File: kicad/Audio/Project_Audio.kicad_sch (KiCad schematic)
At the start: 9 parts, among them U1 PIC32MX170F256B, U2 Audio

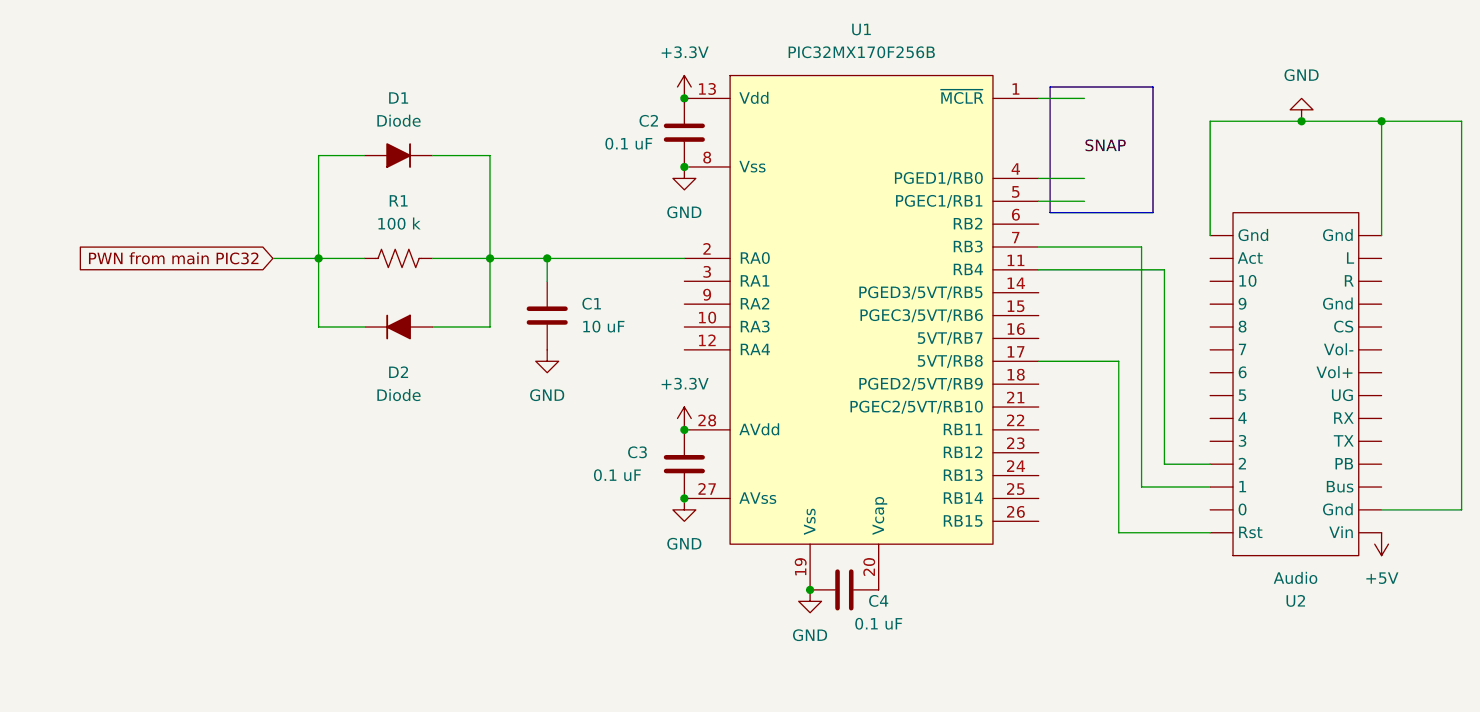
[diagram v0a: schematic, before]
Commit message: Revert to 3d98758
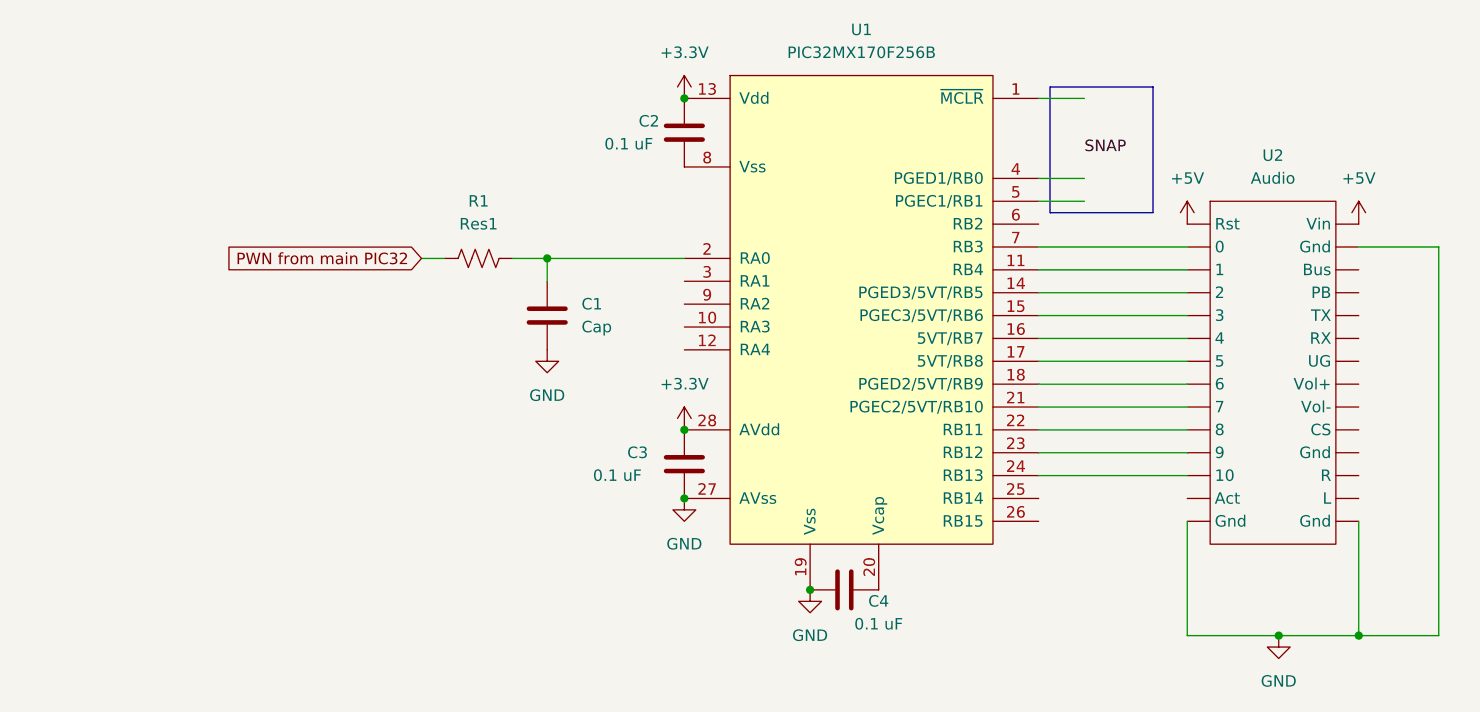
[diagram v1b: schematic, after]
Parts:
- removed D1, D2: Diode, symbol ME218_BaseLib:Diode
- C1: value 10 uF -> Cap
- R1: value 100 k -> Res1
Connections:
- net GND: no longer C2.2, U1.8 (Vss)
- net at U1.14 (PGED3/5VT/RB5): now also U2. (Vol-)
- net at U1.15 (PGEC3/5VT/RB6): now also U2. (Vol-)
- net at U1.16 (5VT/RB7): now also U2. (Vol-)
- net at U1.18 (PGED2/5VT/RB9): now also U2. (Vol-)
- net at U1.21 (PGEC2/5VT/RB10): now also U2. (Vol-)
- net at U1.22 (RB11): now also U2. (Vol-)
- net at U1.23 (RB12): now also U2. (Vol-)
- net at U1.24 (RB13): now also U2. (Vol-)
- new net: C2.2, U1.8 (Vss)
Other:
- moved on the sheet: R1, U2

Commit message: Update audio kicad
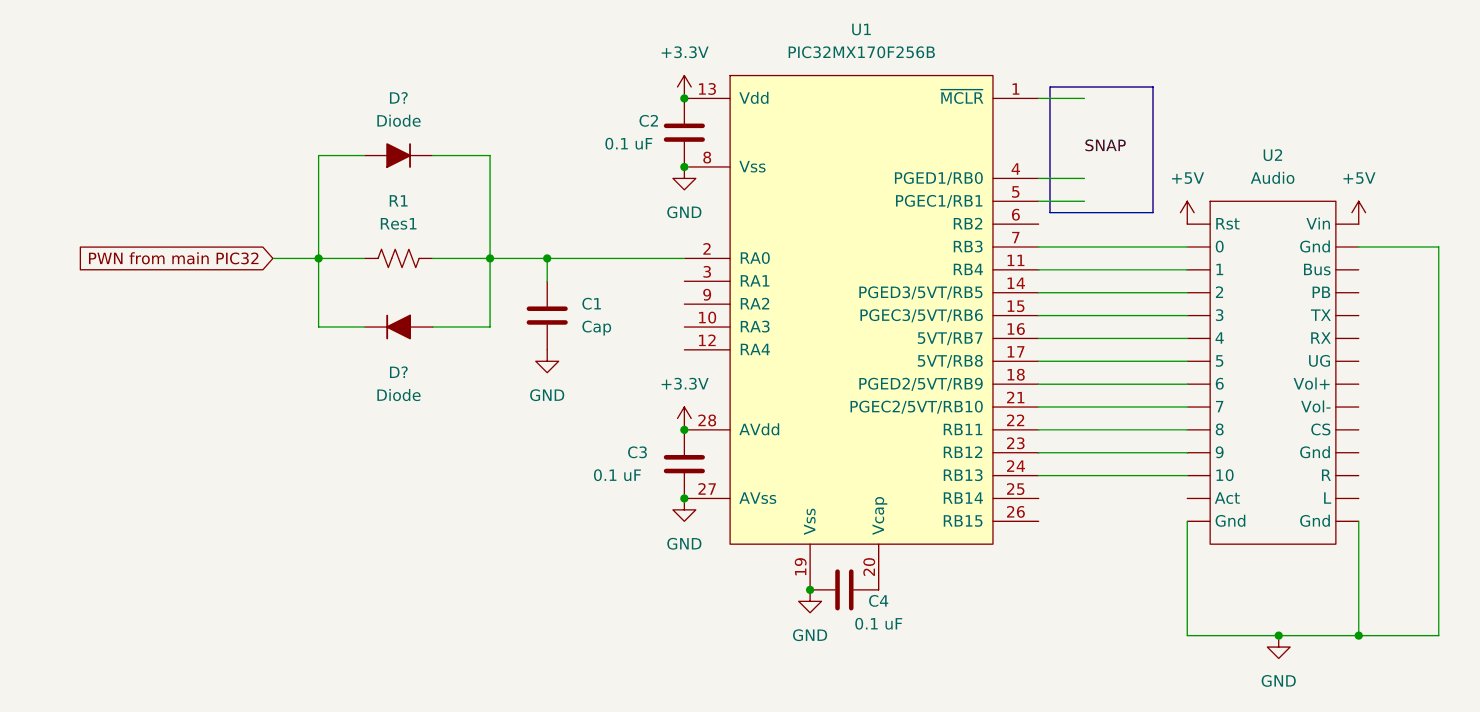
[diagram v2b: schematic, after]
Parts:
- added D? (x2): Diode, symbol ME218_BaseLib:Diode
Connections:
- net GND: now also C2.2, U1.8 (Vss)
- net PWN from main PIC32: now also D?.1 (K), D?.2 (A)
- net at C1.1, R1.2, U1.2 (RA0): now also D?.1 (K), D?.2 (A)
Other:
- moved on the sheet: R1
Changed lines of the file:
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@@
   (junction (at 69.85 85.09) (diameter 0) (color 0 0 0 0)
   )
+  (junction (at 63.5 85.09) (diameter 0) (color 0 0 0 0)
+  )
   (junction (at 85.09 111.76) (diameter 0) (color 0 0 0 0)
   )
@@
   (junction (at 151.13 127) (diameter 0) (color 0 0 0 0)
   )
+  (junction (at 44.45 85.09) (diameter 0) (color 0 0 0 0)
+  )
   (junction (at 85.09 104.14) (diameter 0) (color 0 0 0 0)
   )
@@
   (junction (at 85.09 67.31) (diameter 0) (color 0 0 0 0)
   )
+  (junction (at 85.09 74.93) (diameter 0) (color 0 0 0 0)
+  )
+  (wire (pts (xy 44.45 92.71) (xy 44.45 85.09))
+    (stroke (width 0) (type default) (color 0 0 0 0))
+  )
   (polyline (pts (xy 137.16 80.01) (xy 125.73 80.01))
     (stroke (width 0) (type default) (color 0 0 0 0))
@@
     (stroke (width 0) (type default) (color 0 0 0 0))
   )
-  (wire (pts (xy 55.88 85.09) (xy 58.42 85.09))
+  (wire (pts (xy 39.37 85.09) (xy 44.45 85.09))
     (stroke (width 0) (type default) (color 0 0 0 0))
   )
@@
     (stroke (width 0) (type default) (color 0 0 0 0))
   )
-  (wire (pts (xy 66.04 85.09) (xy 69.85 85.09))
+  (wire (pts (xy 57.15 85.09) (xy 63.5 85.09))
+    (stroke (width 0) (type default) (color 0 0 0 0))
+  )
+  (wire (pts (xy 63.5 85.09) (xy 69.85 85.09))
     (stroke (width 0) (type default) (color 0 0 0 0))
   )
@@
     (stroke (width 0) (type default) (color 0 0 0 0))
   )
+  (wire (pts (xy 49.53 92.71) (xy 44.45 92.71))
+    (stroke (width 0) (type default) (color 0 0 0 0))
+  )
   (wire (pts (xy 124.46 101.6) (xy 140.97 101.6))
     (stroke (width 0) (type default) (color 0 0 0 0))
   )
+  (wire (pts (xy 63.5 73.66) (xy 63.5 85.09))
+    (stroke (width 0) (type default) (color 0 0 0 0))
+  )
   (wire (pts (xy 124.46 91.44) (xy 140.97 91.44))
     (stroke (width 0) (type default) (color 0 0 0 0))
@@
     (stroke (width 0) (type default) (color 0 0 0 0))
   )
+  (wire (pts (xy 63.5 92.71) (xy 63.5 85.09))
+    (stroke (width 0) (type default) (color 0 0 0 0))
+  )
   (wire (pts (xy 124.46 78.74) (xy 129.54 78.74))
     (stroke (width 0) (type default) (color 0 0 0 0))
@@
     (stroke (width 0) (type default) (color 0 0 0 0))
   )
+  (wire (pts (xy 44.45 73.66) (xy 44.45 85.09))
+    (stroke (width 0) (type default) (color 0 0 0 0))
+  )
   (wire (pts (xy 168.91 83.82) (xy 168.91 127))
     (stroke (width 0) (type default) (color 0 0 0 0))
   )
+  (wire (pts (xy 57.15 92.71) (xy 63.5 92.71))
+    (stroke (width 0) (type default) (color 0 0 0 0))
+  )
   (wire (pts (xy 140.97 127) (xy 151.13 127))
     (stroke (width 0) (type default) (color 0 0 0 0))
@@
     (stroke (width 0) (type default) (color 0 0 0 0))
   )
+  (wire (pts (xy 57.15 73.66) (xy 63.5 73.66))
+    (stroke (width 0) (type default) (color 0 0 0 0))
+  )
   (wire (pts (xy 124.46 106.68) (xy 140.97 106.68))
     (stroke (width 0) (type default) (color 0 0 0 0))
   )
   (wire (pts (xy 160.02 114.3) (xy 160.02 127))
+    (stroke (width 0) (type default) (color 0 0 0 0))
+  )
+  (wire (pts (xy 49.53 73.66) (xy 44.45 73.66))
+    (stroke (width 0) (type default) (color 0 0 0 0))
+  )
+  (wire (pts (xy 44.45 85.09) (xy 49.53 85.09))
     (stroke (width 0) (type default) (color 0 0 0 0))
   )
@@
     (effects (font (size 1.27 1.27)) (justify left bottom))
   )
-  (global_label "PWN from main PIC32" (shape input) (at 55.88 85.09 180) (fields_autoplaced)
+  (global_label "PWN from main PIC32" (shape input) (at 39.37 85.09 180) (fields_autoplaced)
     (effects (font (size 1.27 1.27)) (justify right))
-    (property "Intersheet References" "${INTERSHEET_REFS}" (id 0) (at 31.9979 85.0106 0)
+    (property "Intersheet References" "${INTERSHEET_REFS}" (id 0) (at 15.4879 85.0106 0)
       (effects (font (size 1.27 1.27)) (justify right) hide)
     )
@@
     )
     (property "Datasheet" "" (id 3) (at 85.09 67.31 0)
+      (effects (font (size 1.27 1.27)) hide)
+    )
+    (pin "1")
+  )
+  (symbol (lib_id "power:GND") (at 85.09 74.93 0) (unit 1)
+    (in_bom yes) (on_board yes) (fields_autoplaced)
+    (property "Reference" "#PWR?" (id 0) (at 85.09 81.28 0)
+      (effects (font (size 1.27 1.27)) hide)
+    )
+    (property "Value" "GND" (id 1) (at 85.09 80.01 0))
+    (property "Footprint" "" (id 2) (at 85.09 74.93 0)
+      (effects (font (size 1.27 1.27)) hide)
+    )
+    (property "Datasheet" "" (id 3) (at 85.09 74.93 0)
       (effects (font (size 1.27 1.27)) hide)
     )
@@
     )
     (property "Datasheet" "" (id 3) (at 102.87 121.92 0)
+      (effects (font (size 1.27 1.27)) hide)
+    )
+    (pin "1")
+    (pin "2")
+  )
+  (symbol (lib_id "ME218_BaseLib:Diode") (at 53.34 73.66 180) (unit 1)
+    (in_bom yes) (on_board yes) (fields_autoplaced)
+    (property "Reference" "D?" (id 0) (at 53.34 67.31 0))
+    (property "Value" "Diode" (id 1) (at 53.34 69.85 0))
+    (property "Footprint" "" (id 2) (at 53.34 73.66 0)
+      (effects (font (size 1.27 1.27)) hide)
+    )
+    (property "Datasheet" "" (id 3) (at 53.34 73.66 0)
       (effects (font (size 1.27 1.27)) hide)
     )
@@
     (pin "2")
   )
-  (symbol (lib_id "ME218_BaseLib:Res1") (at 62.23 85.09 90) (unit 1)
-    (in_bom yes) (on_board yes) (fields_autoplaced)
-    (property "Reference" "R1" (id 0) (at 62.23 78.74 90))
-    (property "Value" "Res1" (id 1) (at 62.23 81.28 90))
-    (property "Footprint" "" (id 2) (at 62.484 84.074 90)
-      (effects (font (size 1.27 1.27)) hide)
-    )
-    (property "Datasheet" "" (id 3) (at 62.23 85.09 0)
+  (symbol (lib_id "ME218_BaseLib:Diode") (at 53.34 92.71 0) (unit 1)
+    (in_bom yes) (on_board yes)
+    (property "Reference" "D?" (id 0) (at 53.34 97.79 0))
+    (property "Value" "Diode" (id 1) (at 53.34 100.33 0))
+    (property "Footprint" "" (id 2) (at 53.34 92.71 0)
+      (effects (font (size 1.27 1.27)) hide)
+    )
+    (property "Datasheet" "" (id 3) (at 53.34 92.71 0)
+      (effects (font (size 1.27 1.27)) hide)
+    )
+    (pin "1")
+    (pin "2")
+  )
+  (symbol (lib_id "ME218_BaseLib:Res1") (at 53.34 85.09 90) (unit 1)
+    (in_bom yes) (on_board yes) (fields_autoplaced)
+    (property "Reference" "R1" (id 0) (at 53.34 78.74 90))
+    (property "Value" "Res1" (id 1) (at 53.34 81.28 90))
+    (property "Footprint" "" (id 2) (at 53.594 84.074 90)
+      (effects (font (size 1.27 1.27)) hide)
+    )
+    (property "Datasheet" "" (id 3) (at 53.34 85.09 0)
       (effects (font (size 1.27 1.27)) hide)
     )
@@
       (reference "#PWR08") (unit 1) (value "+5V") (footprint "")
     )
+    (path "/39f08828-7987-4a18-a65b-bd8b02efd613"
+      (reference "#PWR?") (unit 1) (value "GND") (footprint "")
+    )
     (path "/9936a45c-d9ed-4757-8965-fef1371db57d"
       (reference "C1") (unit 1) (value "Cap") (footprint "")
@@
       (reference "C4") (unit 1) (value "0.1 uF") (footprint "")
     )
+    (path "/919e989e-be09-45ed-a3b6-56c8307106d6"
+      (reference "D?") (unit 1) (value "Diode") (footprint "")
+    )
+    (path "/d73ebf58-e339-44ac-b350-416d66c9dcea"
+      (reference "D?") (unit 1) (value "Diode") (footprint "")
+    )
     (path "/df0418e5-cc6d-4e9d-b411-2c9742773b02"
